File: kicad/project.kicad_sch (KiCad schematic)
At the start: 15 parts, among them IC1A Conn_02x08_Counter_Clockwise, IC1B Conn_02x08_Counter_Clockwise, Q1 AO3402, Q2 AO3401, SW1 RotaryEncoder_Switch, U2 I2C 0.91 OLED

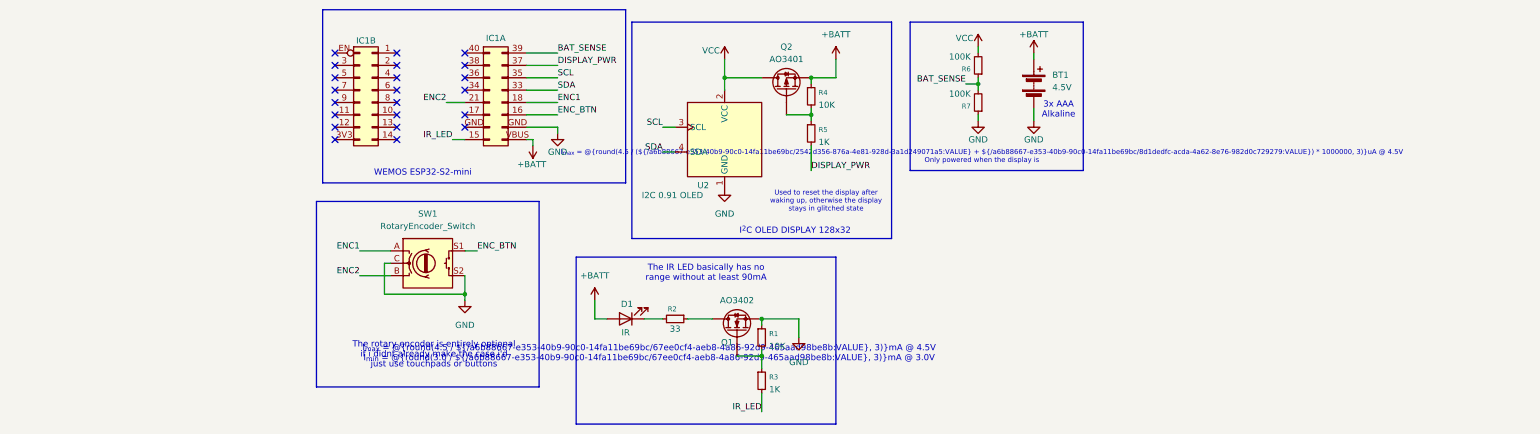
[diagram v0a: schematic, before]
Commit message: Updating the schematic with footprint and symbol
Tiny weaks to pin assignment
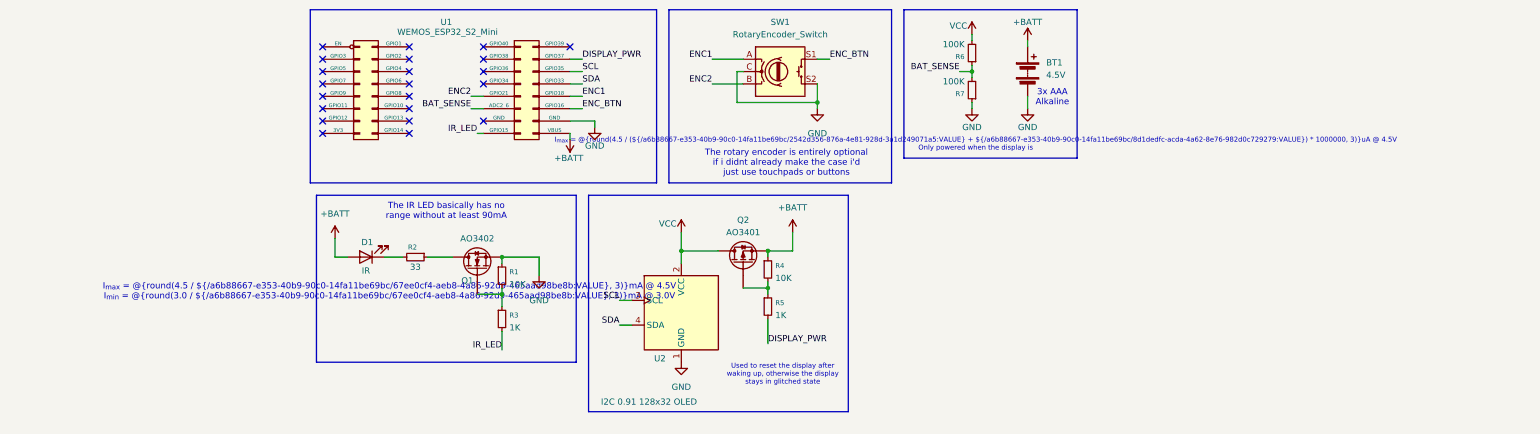
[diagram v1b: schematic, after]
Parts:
- removed IC1A, IC1B: Conn_02x08_Counter_Clockwise, symbol Connector_Generic:Conn_02x08_Counter_Clockwise
- added U1: WEMOS_ESP32_S2_Mini, library:WEMOS_S2_mini, symbol library:WEMOS_ESP32_S2_Mini
- BT1: footprint (none) -> Connector_PinHeader_2.54mm:PinHeader_1x02_P2.54mm_Vertical
- R1, R2, R3, R4, R5, R6, R7: footprint (none) -> Resistor_THT:R_Axial_DIN0207_L6.3mm_D2.5mm_P10.16mm_Horizontal
- U2: value I2C 0.91 OLED -> I2C 0.91 128x32 OLED
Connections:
- net +BATT: now also U1.47 (VBUS)
- net BAT_SENSE: now also U1.17 (GPIO17)
- net DISPLAY_PWR: now also U1.37 (GPIO37)
- net ENC1: now also U1.18 (GPIO18)
- net ENC2: now also U1.21 (GPIO21)
- net ENC_BTN: now also U1.16 (GPIO16)
- net GND: now also U1.48 (GND)
- net IR_LED: now also U1.15 (GPIO15)
- net SCL: now also U1.35 (GPIO35)
- net SDA: now also U1.33 (GPIO33)
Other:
- note removed: "I^{2}C OLED DISPLAY 128x32"
- note removed: "WEMOS ESP32-S2-mini"
- moved on the sheet: BT1, D1, Q1, Q2, R1, R2, R3, R4, R5, R6, R7, SW1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
